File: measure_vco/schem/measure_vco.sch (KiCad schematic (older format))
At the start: 45 parts, among them Q1 2N7000, Q3 1/2 BCM847, Q4 1/2 BCM847, U1 LM324, U2 LM324, U3 LM324, U4 MCP4822, U5 LM317L_TO92, U6 LM324, U7 LM324, U8 LM324

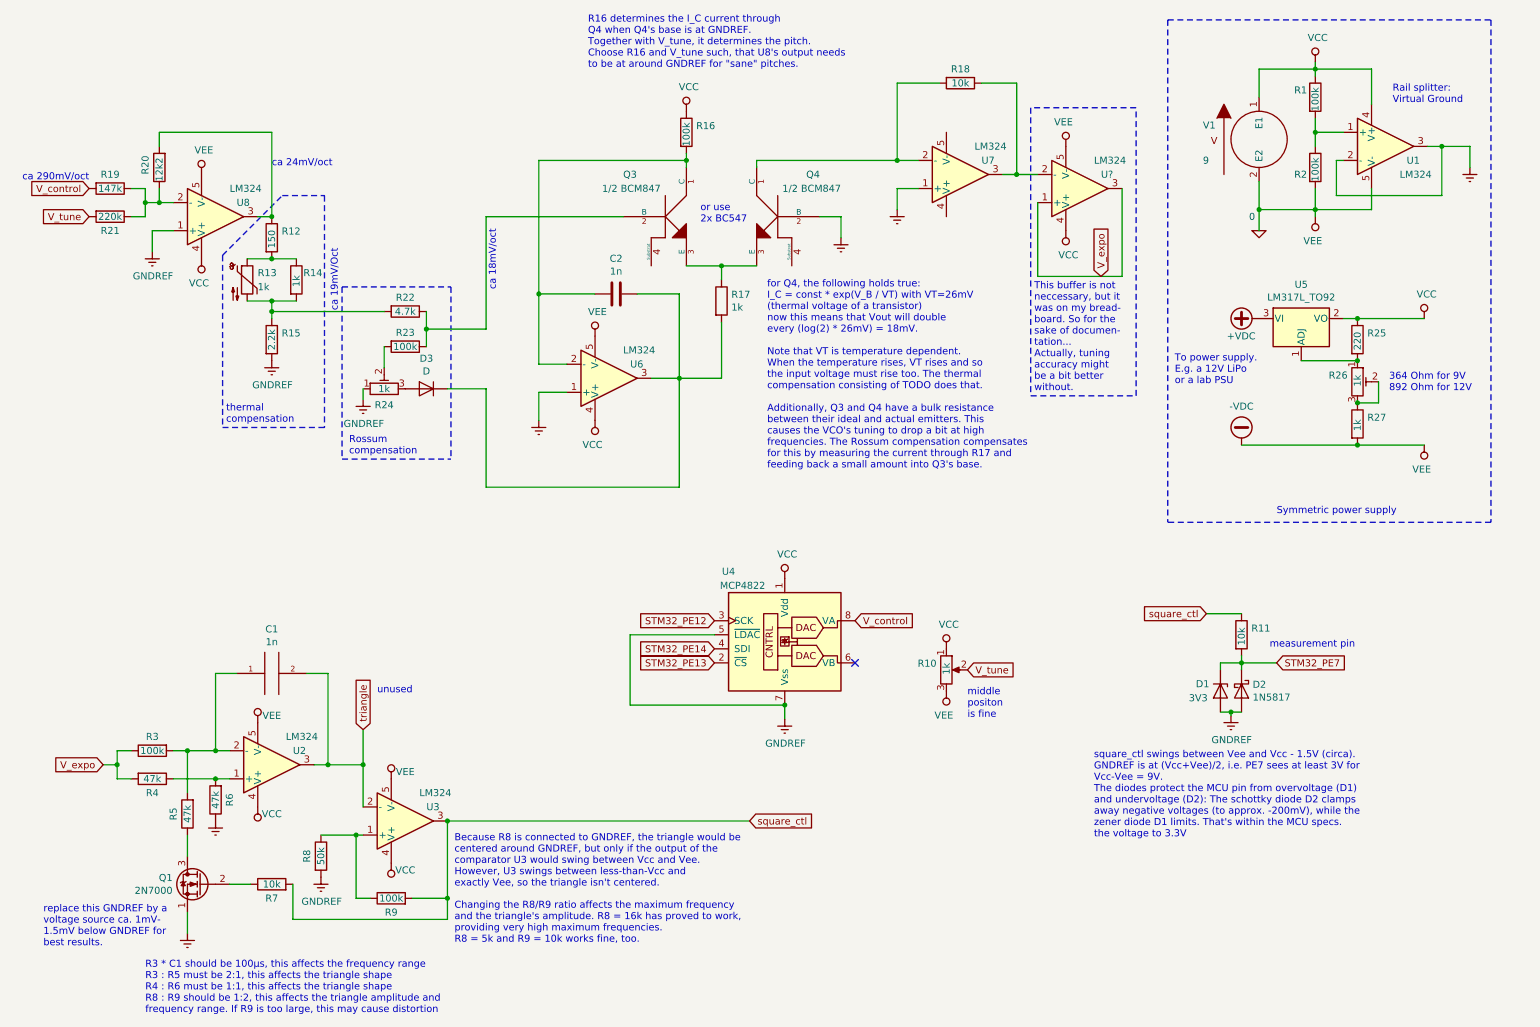
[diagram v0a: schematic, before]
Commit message: update measure_vco schematics
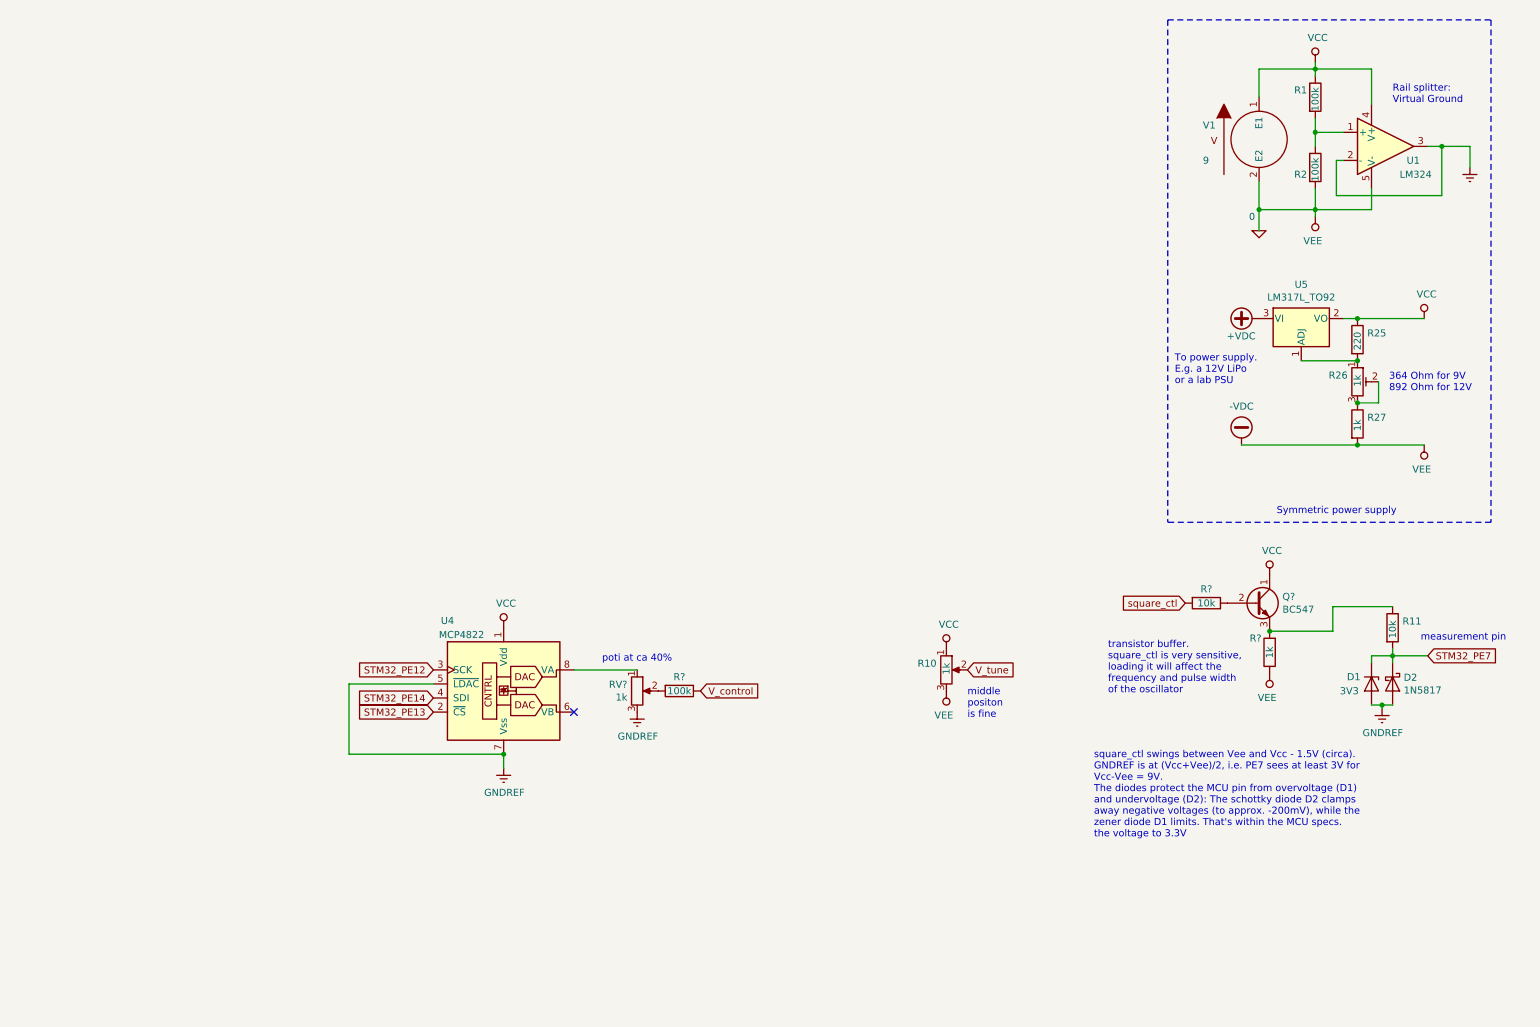
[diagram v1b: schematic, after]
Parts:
- removed C1: 1n, symbol pspice:C
- removed C2: 1n, symbol Device:C
- removed D3: D, symbol Device:D
- removed Q1: 2N7000, Package_TO_SOT_THT:TO-92_Inline, symbol Transistor_FET:2N7000
- removed Q3, Q4: 1/2 BCM847, symbol pspice:QNPN
- removed R12: 150, symbol Device:R
- removed R13: 1k, symbol Device:Thermistor_NTC
- removed R14, R17: 1k, symbol Device:R
- removed R15: 2.2k, symbol Device:R
- removed R16, R23, R3, R9: 100k, symbol Device:R
- removed R18, R7: 10k, symbol Device:R
- removed R19: 147k, symbol Device:R
- removed R20: 12k2, symbol Device:R
- removed R21: 220k, symbol Device:R
- removed R22: 4.7k, symbol Device:R
- removed R24: 1k, symbol Device:R_POT_TRIM
- removed R4, R5, R6: 47k, symbol Device:R
- removed R8: 50k, symbol Device:R
- removed U2, U3, U6, U7, U8, U?: LM324, symbol pspice:OPAMP
- added Q?: BC547, Package_TO_SOT_THT:TO-92_Inline, symbol Transistor_BJT:BC547
- added R?: 10k, symbol Device:R
- added R?: 1k, symbol Device:R
- added R?: 100k, symbol Device:R
- added RV?: 1k, symbol Device:R_POT
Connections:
- net -VDC: now also R?.1
- net GNDREF: now also RV?.3
- net VCC: now also Q?.1 (C)
- net V_control: now also R?.1; no longer U4.8 (VA)
- net square_ctl: now also R?.2; no longer R11.1
- new net: RV?.1, U4.8 (VA)
- new net: Q?.3 (E), R11.1, R?.2
- new net: Q?.2 (B), R?.1
- new net: R?.2, RV?.2
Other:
- note added: "poti at ca 40%"
- note added: "transistor buffer.\nsquare_ctl is very sensitive,\nloading it will affect the\nfrequency and pulse width\nof the oscillator"
- note removed: "Because R8 is connected to GNDREF, the triangle would be\ncentered around GNDREF, but only if the output of the\ncomparator U3 would swing between Vcc and Vee.\nHowever, U3 swings between less-than-Vcc and\nexactly Vee, so the triangle isn't centered."
- note removed: "Changing the R8/R9 ratio affects the maximum frequency\nand the triangle's amplitude. R8 = 16k has proved to work,\nproviding very high maximum frequencies.\nR8 = 5k and R9 = 10k works fine, too."
- note removed: "R16 determines the I_C current through\nQ4 when Q4's base is at GNDREF.\nTogether with V_tune, it determines the pitch.\nChoose R16 and V_tune such, that U8's output needs\nto be at around GNDREF for "sane" pitches."
- note removed: "R3 * C1 should be 100µs, this affects the frequency range\nR3 : R5 must be 2:1, this affects the triangle shape\nR4 : R6 must be 1:1, this affects the triangle shape\nR8 : R9 should be 1:2, this affects the triangle amplitude and\nfrequency range. If R9 is too large, this may cause distortion"
- note removed: "Rossum\ncompensation"
- note removed: "This buffer is not\nneccessary, but it\nwas on my bread-\nboard. So for the\nsake of documen-\ntation...\nActually, tuning\naccuracy might\nbe a bit better\nwithout."
- note removed: "ca 18mV/oct"
- note removed: "ca 19mV/Oct"
- note removed: "ca 24mV/oct"
- note removed: "ca 290mV/oct"
- note removed: "for Q4, the following holds true:\nI_C = const * exp(V_B / VT) with VT=26mV\n(thermal voltage of a transistor)\nnow this means that Vout will double\nevery (log(2) * 26mV) = 18mV.\n\nNote that VT is temperature dependent.\nWhen the temperature rises, VT rises and so\nthe input voltage must rise too. The thermal\ncompensation consisting of TODO does that.\n\nAdditionally, Q3 and Q4 have a bulk res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"
- note removed: "or use\n2x BC547"
- note removed: "replace this GNDREF by a\nvoltage source ca. 1mV-\n1.5mV below GNDREF for\nbest results."
- note removed: "thermal\ncompensation"
- note removed: "unused"
- moved on the sheet: D1, D2, R11, U4
